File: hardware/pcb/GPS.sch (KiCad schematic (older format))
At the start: 10 parts, among them U13 u-blox_max-7c/q, U14 MAX2659

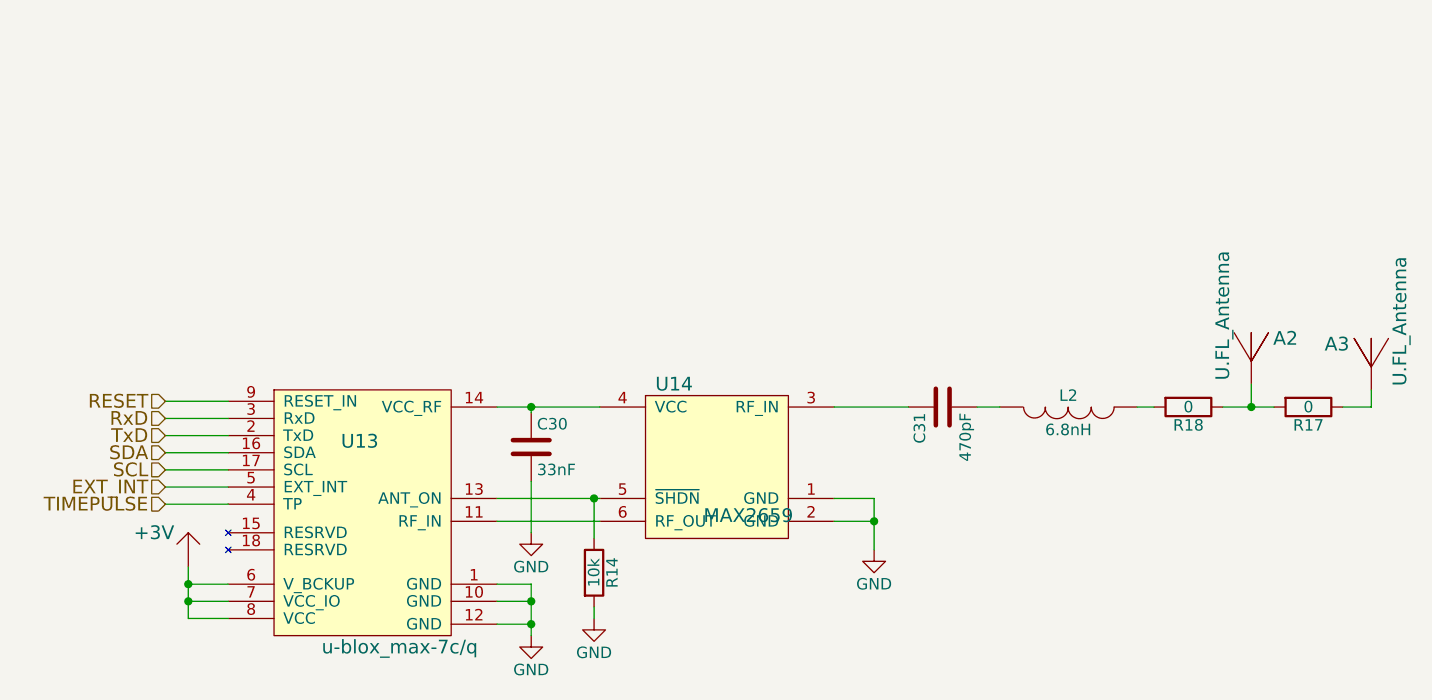
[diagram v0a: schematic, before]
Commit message: pre-net import
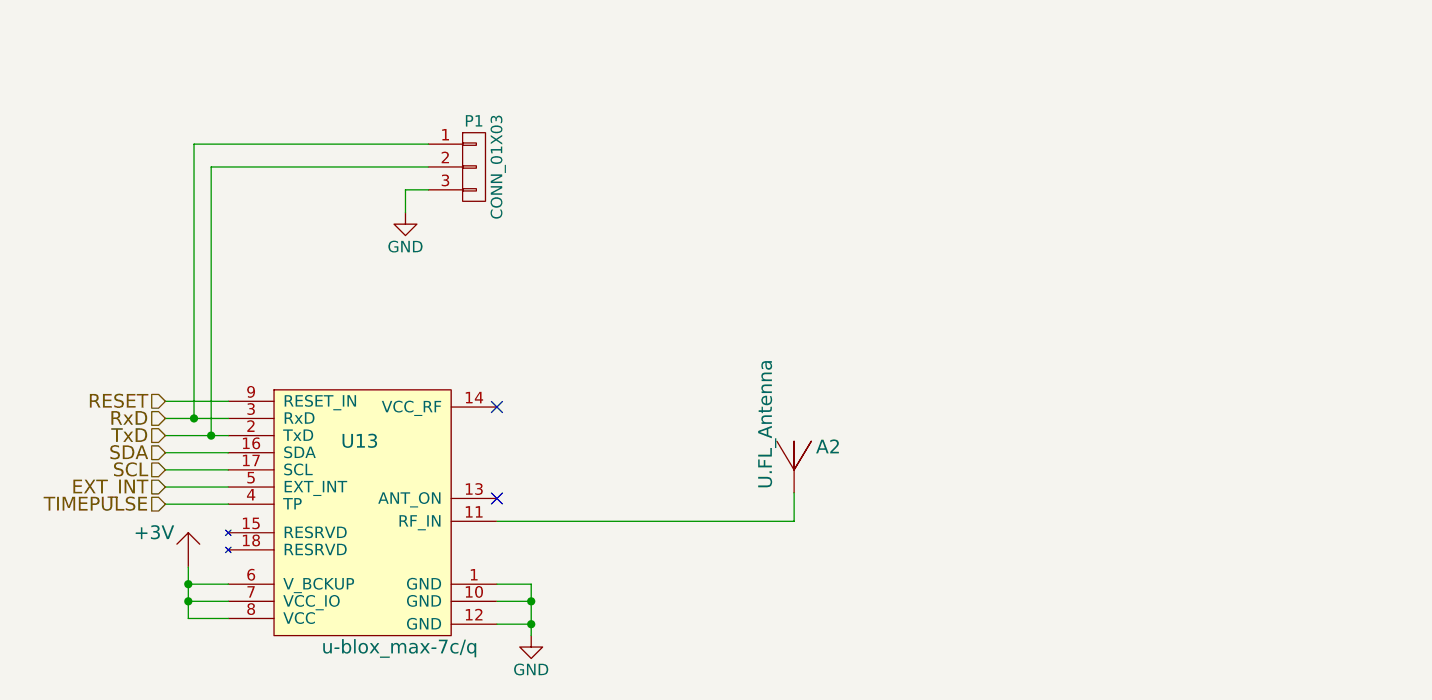
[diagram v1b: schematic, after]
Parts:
- removed A3: U.FL_Antenna, aero:Chip_Antenna_W3011A, symbol U.FL_Antenna
- removed C30: 33nF, Capacitors_SMD:C_0402, symbol C
- removed C31: 470pF, Capacitors_SMD:C_0402, symbol C
- removed L2: 6.8nH, Capacitors_SMD:C_0402, symbol INDUCTOR
- removed R14: 10k, Resistors_SMD:R_0402, symbol R
- removed R17, R18: 0, Resistors_SMD:R_0402, symbol R
- removed U14: MAX2659, aero:6-µDFN, symbol MAX2659-RESCUE-aero
- added P1: CONN_01X03, Pin_Headers:Pin_Header_Straight_1x03, symbol CONN_01X03
- A2: footprint aero:U.FL -> aero:CGGP.25.4.A.02
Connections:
- net GND: now also P1.3 (P3)
- net RxD: now also P1.1 (P1)
- net TxD: now also P1.2 (P2)
- net at U13.11 (RF_IN): now also A2.1 (RF_IN)
- no-connect marks 0 -> 2
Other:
- moved on the sheet: A2
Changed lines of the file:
@@
 $EndDescr
-$Comp
-L MAX2659-RESCUE-aero U14
-U 1 1 55B6C335
-P 6750 3750
-AR Path="/55B6C335" Ref="U14"  Part="1"
-AR Path="/55B6C26A/55B6C335" Ref="U14"  Part="1"
-F 0 "U14" H 6550 4025 60  0000 C CNN
-F 1 "MAX2659" H 6875 3450 60  0000 C CNN
-F 2 "aero:6-µDFN" H 6700 3450 60  0001 C CNN
-F 3 "" H 6700 3450 60  0000 C CNN
-	1    6750 3750
-	1    0    0    -1
-$EndComp
-$Comp
-L C C31
-U 1 1 55B6C37F
-P 7725 3575
-F 0 "C31" H 7750 3675 50  0000 L CNN
-F 1 "470pF" H 7750 3475 50  0000 L CNN
-F 2 "Capacitors_SMD:C_0402" H 7763 3425 30  0001 C CNN
-F 3 "" H 7725 3575 60  0000 C CNN
-	1    7725 3575
-	0    -1   1    0
-$EndComp
-$Comp
-L INDUCTOR L2
-U 1 1 55B6C3BB
-P 8275 3575
-F 0 "L2" V 8225 3575 50  0000 C CNN
-F 1 "6.8nH" V 8375 3575 50  0000 C CNN
-F 2 "Capacitors_SMD:C_0402" H 8275 3575 60  0001 C CNN
-F 3 "" H 8275 3575 60  0000 C CNN
-	1    8275 3575
-	0    -1   1    0
-$EndComp
 $Comp
 L U.FL_Antenna A2
 U 1 1 55B6C93F
-P 9075 3475
-F 0 "A2" H 8925 3675 60  0000 C CNN
-F 1 "U.FL_Antenna" V 9200 3775 60  0000 C CNN
-F 2 "aero:U.FL" H 9075 3475 60  0001 C CNN
-F 3 "" H 9075 3475 60  0000 C CNN
-	1    9075 3475
+P 7075 3950
+F 0 "A2" H 6925 4150 60  0000 C CNN
+F 1 "U.FL_Antenna" V 7200 4250 60  0000 C CNN
+F 2 "aero:CGGP.25.4.A.02" H 7075 3950 60  0001 C CNN
+F 3 "" H 7075 3950 60  0000 C CNN
+	1    7075 3950
 	-1   0    0    -1
 $EndComp
@@
 F 3 "" H 5925 4575 60  0000 C CNN
 	1    5925 4575
-	1    0    0    -1
-$EndComp
-$Comp
-L GND #PWR056
-U 1 1 55B7095D
-P 6200 4500
-F 0 "#PWR056" H 6200 4250 50  0001 C CNN
-F 1 "GND" H 6200 4350 50  0000 C CNN
-F 2 "" H 6200 4500 60  0000 C CNN
-F 3 "" H 6200 4500 60  0000 C CNN
-	1    6200 4500
-	1    0    0    -1
-$EndComp
-$Comp
-L R R14
-U 1 1 55B7097D
-P 6200 4300
-F 0 "R14" V 6280 4300 50  0000 C CNN
-F 1 "10k" V 6200 4300 50  0000 C CNN
-F 2 "Resistors_SMD:R_0402" V 6130 4300 30  0001 C CNN
-F 3 "" H 6200 4300 30  0000 C CNN
-	1    6200 4300
 	1    0    0    -1
 $EndComp
@@
 RESET
 $Comp
-L +3V #PWR057
+L +3V #PWR056
 U 1 1 55B708B7
 P 4425 4275
-F 0 "#PWR057" H 4425 4175 60  0001 C CNN
+F 0 "#PWR056" H 4425 4175 60  0001 C CNN
 F 1 "+3V" H 4275 4425 60  0000 C CNN
 F 2 "" H 4425 4275 60  0000 C CNN
@@
 	1    0    0    -1
 $EndComp
-$Comp
-L C C30
-U 1 1 55B6CB58
-P 5925 3750
-F 0 "C30" H 5950 3850 50  0000 L CNN
-F 1 "33nF" H 5950 3650 50  0000 L CNN
-F 2 "Capacitors_SMD:C_0402" H 5963 3600 30  0001 C CNN
-F 3 "" H 5925 3750 60  0000 C CNN
-	1    5925 3750
-	1    0    0    -1
-$EndComp
-$Comp
-L GND #PWR058
-U 1 1 55BA5DAD
-P 5925 4125
-F 0 "#PWR058" H 5925 3875 50  0001 C CNN
-F 1 "GND" H 5925 3975 50  0000 C CNN
-F 2 "" H 5925 4125 60  0000 C CNN
-F 3 "" H 5925 4125 60  0000 C CNN
-	1    5925 4125
-	1    0    0    -1
-$EndComp
-$Comp
-L GND #PWR059
-U 1 1 55BA62A6
-P 7425 4200
-F 0 "#PWR059" H 7425 3950 50  0001 C CNN
-F 1 "GND" H 7425 4050 50  0000 C CNN
-F 2 "" H 7425 4200 60  0000 C CNN
-F 3 "" H 7425 4200 60  0000 C CNN
-	1    7425 4200
-	1    0    0    -1
-$EndComp
-$Comp
-L R R17
-U 1 1 55C545D1
-P 9325 3575
-F 0 "R17" V 9405 3575 50  0000 C CNN
-F 1 "0" V 9325 3575 50  0000 C CNN
-F 2 "Resistors_SMD:R_0402" V 9255 3575 30  0001 C CNN
-F 3 "" H 9325 3575 30  0000 C CNN
-	1    9325 3575
-	0    1    1    0
-$EndComp
-$Comp
-L U.FL_Antenna A3
-U 1 1 55C54C8E
-P 9600 3500
-F 0 "A3" H 9450 3700 60  0000 C CNN
-F 1 "U.FL_Antenna" V 9725 3800 60  0000 C CNN
-F 2 "aero:Chip_Antenna_W3011A" H 9600 3500 60  0001 C CNN
-F 3 "" H 9600 3500 60  0000 C CNN
-	1    9600 3500
-	1    0    0    -1
-$EndComp
-Wire Wire Line
-	7250 3575 7575 3575
-Wire Wire Line
-	7875 3575 7975 3575
-Wire Wire Line
-	9600 3575 9600 3500
-Wire Wire Line
-	6200 4450 6200 4500
 Wire Wire Line
 	4600 3550 4325 3550
@@
 Connection ~ 5925 4525
 Wire Wire Line
-	5775 4075 6225 4075
-Wire Wire Line
-	6225 3975 5775 3975
-Wire Wire Line
-	5775 3575 6225 3575
-Wire Wire Line
-	5925 3575 5925 3600
-Connection ~ 5925 3575
-Wire Wire Line
-	5925 3900 5925 4125
-Wire Wire Line
-	6200 4150 6200 3975
-Connection ~ 6200 3975
-Wire Wire Line
-	7250 3975 7425 3975
-Wire Wire Line
-	7425 3975 7425 4200
-Wire Wire Line
-	7250 4075 7425 4075
-Connection ~ 7425 4075
-Wire Wire Line
-	8950 3575 9175 3575
-Wire Wire Line
-	9475 3575 9600 3575
-Wire Wire Line
-	9075 3475 9075 3575
-Connection ~ 9075 3575
+	5775 4075 7075 4075
 $Comp
-L R R18
-U 1 1 55CD5A0B
-P 8800 3575
-F 0 "R18" V 8880 3575 50  0000 C CNN
-F 1 "0" V 8800 3575 50  0000 C CNN
-F 2 "Resistors_SMD:R_0402" V 8730 3575 30  0001 C CNN
-F 3 "" H 8800 3575 30  0000 C CNN
-	1    8800 3575
-	0    1    1    0
+L CONN_01X03 P1
+U 1 1 5612ECE3
+P 5675 2525
+F 0 "P1" H 5675 2725 50  0000 C CNN
+F 1 "CONN_01X03" V 5775 2525 50  0000 C CNN
+F 2 "Pin_Headers:Pin_Header_Straight_1x03" H 5675 2525 60  0001 C CNN
+F 3 "" H 5675 2525 60  0000 C CNN
+	1    5675 2525
+	1    0    0    -1
 $EndComp
 Wire Wire Line
-	8575 3575 8650 3575
+	4450 3625 4450 2425
+Wire Wire Line
+	4450 2425 5475 2425
+Connection ~ 4450 3625
+Wire Wire Line
+	4525 3700 4525 2525
+Wire Wire Line
+	4525 2525 5475 2525
+Connection ~ 4525 3700
+$Comp
+L GND #PWR057
+U 1 1 5612EDCC
+P 5375 2725
+F 0 "#PWR057" H 5375 2475 50  0001 C CNN
+F 1 "GND" H 5375 2575 50  0000 C CNN
+F 2 "" H 5375 2725 60  0000 C CNN
+F 3 "" H 5375 2725 60  0000 C CNN
+	1    5375 2725
+	1    0    0    -1
+$EndComp
+Wire Wire Line
+	5475 2625 5375 2625
+Wire Wire Line
+	5375 2625 5375 2725
+NoConn ~ 5775 3575
+NoConn ~ 5775 3975
+Wire Wire Line
+	7075 4075 7075 3950
 $EndSCHEMATC

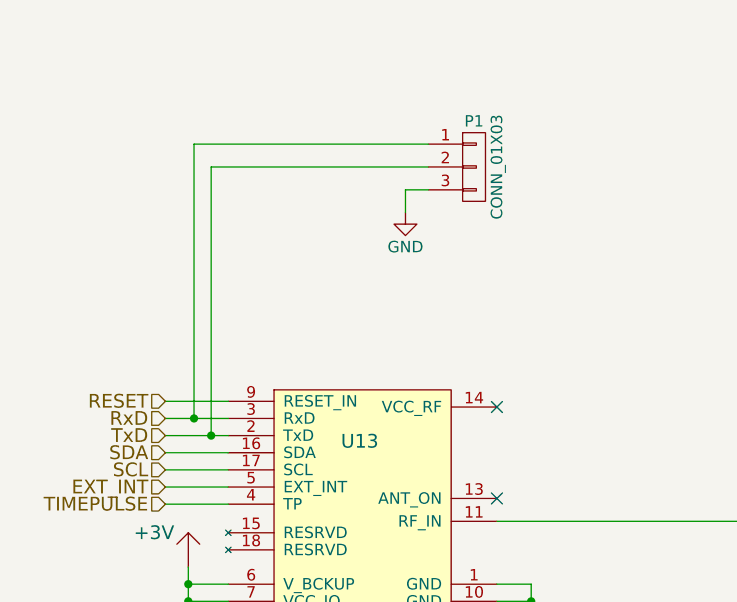
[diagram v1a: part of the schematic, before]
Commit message: intermediate
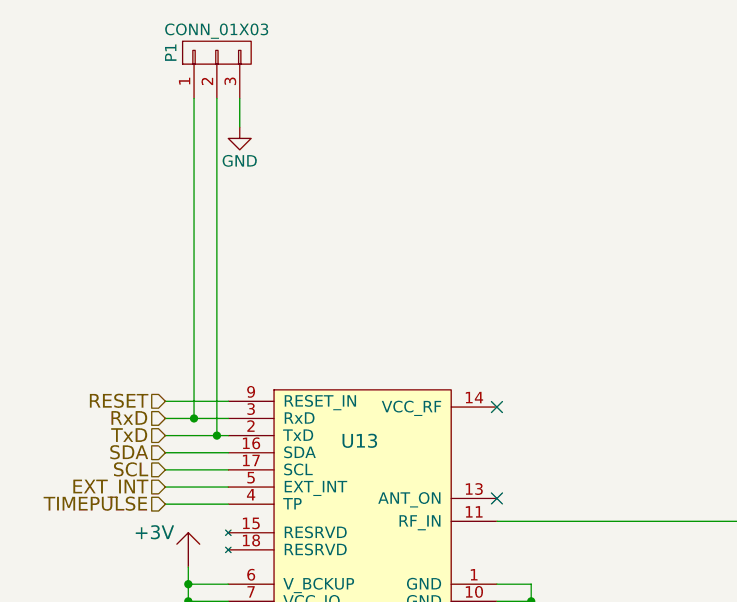
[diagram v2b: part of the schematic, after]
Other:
- moved on the sheet: P1
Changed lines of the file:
@@
 L CONN_01X03 P1
 U 1 1 5612ECE3
-P 5675 2525
-F 0 "P1" H 5675 2725 50  0000 C CNN
-F 1 "CONN_01X03" V 5775 2525 50  0000 C CNN
-F 2 "Pin_Headers:Pin_Header_Straight_1x03" H 5675 2525 60  0001 C CNN
-F 3 "" H 5675 2525 60  0000 C CNN
-	1    5675 2525
-	1    0    0    -1
+P 4550 2025
+F 0 "P1" H 4550 2225 50  0000 C CNN
+F 1 "CONN_01X03" V 4650 2025 50  0000 C CNN
+F 2 "Pin_Headers:Pin_Header_Straight_1x03" H 4550 2025 60  0001 C CNN
+F 3 "" H 4550 2025 60  0000 C CNN
+	1    4550 2025
+	0    -1   -1   0
 $EndComp
 Wire Wire Line
-	4450 3625 4450 2425
-Wire Wire Line
-	4450 2425 5475 2425
+	4450 2225 4450 3625
 Connection ~ 4450 3625
-Wire Wire Line
-	4525 3700 4525 2525
-Wire Wire Line
-	4525 2525 5475 2525
-Connection ~ 4525 3700
 $Comp
 L GND #PWR057
 U 1 1 5612EDCC
-P 5375 2725
-F 0 "#PWR057" H 5375 2475 50  0001 C CNN
-F 1 "GND" H 5375 2575 50  0000 C CNN
-F 2 "" H 5375 2725 60  0000 C CNN
-F 3 "" H 5375 2725 60  0000 C CNN
-	1    5375 2725
+P 4650 2350
+F 0 "#PWR057" H 4650 2100 50  0001 C CNN
+F 1 "GND" H 4650 2200 50  0000 C CNN
+F 2 "" H 4650 2350 60  0000 C CNN
+F 3 "" H 4650 2350 60  0000 C CNN
+	1    4650 2350
 	1    0    0    -1
 $EndComp
-Wire Wire Line
-	5475 2625 5375 2625
-Wire Wire Line
-	5375 2625 5375 2725
 NoConn ~ 5775 3575
 NoConn ~ 5775 3975
 Wire Wire Line
 	7075 4075 7075 3950
+Wire Wire Line
+	4550 2225 4550 3700
+Connection ~ 4550 3700
+Wire Wire Line
+	4650 2225 4650 2350
 $EndSCHEMATC
